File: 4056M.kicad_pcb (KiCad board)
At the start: 2 copper layers, 21.1 x 16 mm, 25 parts, among them J1 VBUS, J2 GND, J3 Conn_01x02_MountingPin, J4 3V3, J5 state, J6 measure, Q1 3401, Q2 8050, Q3 3401, U1 TC4056A, U2 ME6210AXXM3, U3 ME6210AXXP

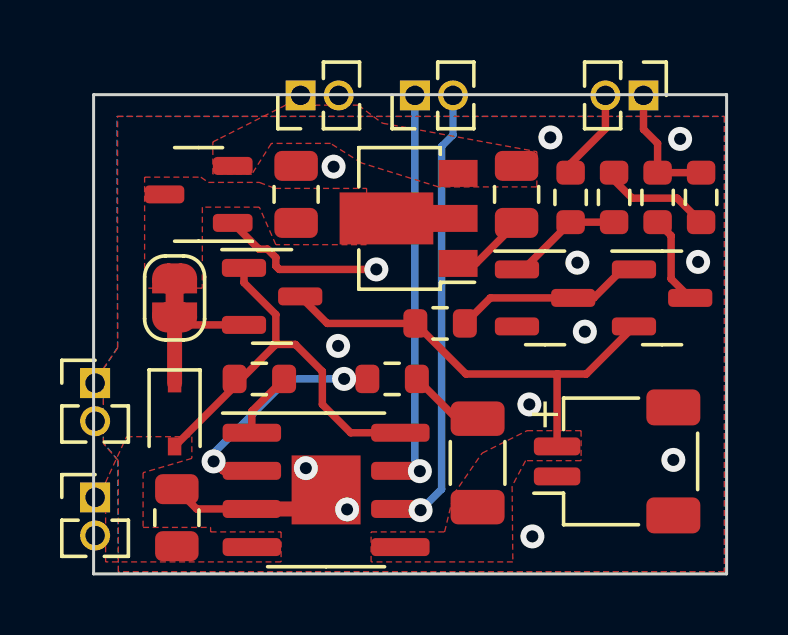
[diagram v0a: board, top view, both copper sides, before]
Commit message: New version
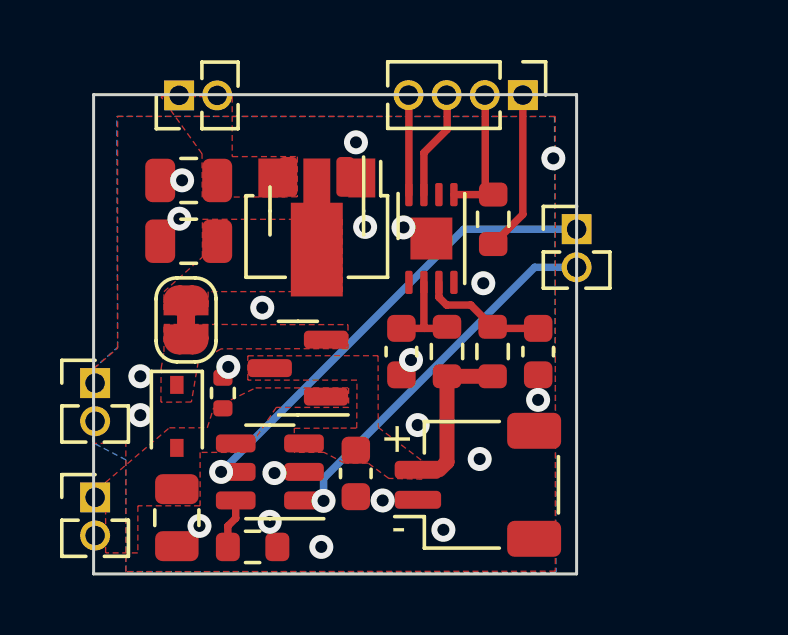
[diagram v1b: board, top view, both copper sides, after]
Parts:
- removed Q2: 8050, Package_TO_SOT_SMD:SOT-23
- removed Q3: 3401, Package_TO_SOT_SMD:SOT-23
- removed R7: 4.7K, Resistor_SMD:R_0603_1608Metric
- removed R8: 1K, Resistor_SMD:R_0603_1608Metric
- added C5: 1uF, Capacitor_SMD:C_0603_1608Metric, F.Cu at (120.3, 84.1)
- added C6: 1uF, Capacitor_SMD:C_0603_1608Metric, F.Cu at (124.9, 84.1)
- added U4: CW2015, Package_DFN_QFN:TDFN-8-1EP_3x2mm_P0.5mm_EP1.4x1.4mm, F.Cu at (121.3, 80.3)
- C2: footprint Capacitor_SMD:C_1206_3216Metric -> Capacitor_SMD:C_0603_1608Metric
- J6: value measure -> Conn_01x04; footprint Connector_PinHeader_1.27mm:PinHeader_1x02_P1.27mm_Vertical -> Connector_PinHeader_1.27mm:PinHeader_1x04_P1.27mm_Vertical
- R2: footprint Resistor_SMD:R_0603_1608Metric -> Resistor_SMD:R_0402_1005Metric
- R4: value 1K -> 470R
- R5: value 100K -> 100R
- R6: value 10K -> 4.7K
- U1: value TC4056A -> TP4057; footprint Package_SO:HSOP-8-1EP_3.9x4.9mm_P1.27mm_EP2.3x2.3mm -> Package_TO_SOT_SMD:SOT-23-6
- moved C4 10.9 mm to (113.2, 78.4), turned to 0 degrees
- moved R1 7.28 mm to (115.3, 90.6)
- moved J5 7.00 mm to (126.2, 80.0), turned to 0 degrees
- moved R4 6.59 mm to (121.8, 84.1), turned to 90 degrees
- moved R5 6.54 mm to (123.3, 84.1)
- moved J3 4.71 mm to (122.9, 88.5)
- moved C2 4.08 mm to (118.8, 88.2), turned to 90 degrees
- moved J4 4.05 mm to (112.9, 75.5)
- moved J6 4.02 mm to (124.4, 75.5)
- moved U2 3.98 mm to (117.5, 79.4), turned to -90 degrees
- moved C3 3.91 mm to (113.2, 80.4), turned to 0 degrees
- moved R6 3.90 mm to (123.4, 79.7), turned to 90 degrees
- moved U3 3.07 mm to (117.5, 80.0), turned to -90 degrees
- moved Q1 2.54 mm to (116.9, 84.6), turned to 180 degrees
- moved U1 1.97 mm to (115.9, 88.1), turned to 180 degrees
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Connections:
- J5 pad 1: /CHRG -> /STDBY
- J5 pad 2: /STDBY -> /CHRG
- J6 pad 1: /ADC -> /PS
- J6 pad 2: /IO -> /ALRT
- R4 pad 1: /IO -> +BATT
- R4 pad 2: Net-(Q2-Pad1) -> Net-(C5-Pad2)
- R5 pad 1: Net-(Q2-Pad1) -> +BATT
- R5 pad 2: -BATT -> Net-(C6-Pad1)
- R6 pad 1: +BATT -> /PS
- R6 pad 2: Net-(Q2-Pad3) -> /ALRT
- U1 pad 1: -BATT -> /CHRG
- U1 pad 2: Net-(R1-Pad2) -> -BATT
- U1 pad 3: -BATT -> +BATT
- U1 pad 5: +BATT -> /STDBY
- U1 pad 6: /STDBY -> Net-(R1-Pad2)
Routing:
- net -BATT: track 22.6 -> 0.00 mm, vias 13 -> 21
- net VBUS: track 13.9 -> 0.00 mm
- net +BATT: track 15.3 -> 5.46 mm
- net Net-(Q2-Pad3): track 6.38 -> 0.00 mm
- net Net-(R1-Pad2): track 7.83 -> 1.66 mm, vias 2 -> 0
- net /PS: track 0.00 -> 5.26 mm
- net Net-(D1-Pad1): track 4.62 -> 0.00 mm
- net /ALRT: track 0.00 -> 4.25 mm
- net Net-(C6-Pad1): track 0.00 -> 4.24 mm
- net /ADC: track 4.22 -> 0.00 mm
- net Net-(Q2-Pad1): track 3.89 -> 0.00 mm
- net /SCL: track 0.00 -> 3.53 mm
- net /SDA: track 0.00 -> 3.21 mm
- net Net-(C5-Pad2): track 0.00 -> 3.08 mm
- net /IO: track 3.06 -> 0.00 mm
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- added copper zone on F.Cu, net Net-(D1-Pad1)
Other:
- board size 21.1 x 16 mm -> 16.1 x 16 mm
- board text added: "-"
- board text added: "Power Module"
